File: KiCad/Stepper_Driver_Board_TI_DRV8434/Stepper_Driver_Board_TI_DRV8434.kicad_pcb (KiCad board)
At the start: 4 copper layers, 25 parts, among them J1 Motor Connect, J2 PWR & DATA Connect, J3 Battery Connect, SW1 SW_SPDT_MSM, SW2 SW_SPDT_MSM, U1 DRV8434PWPR, U2 PC817, U4 6N137, U6 PC817

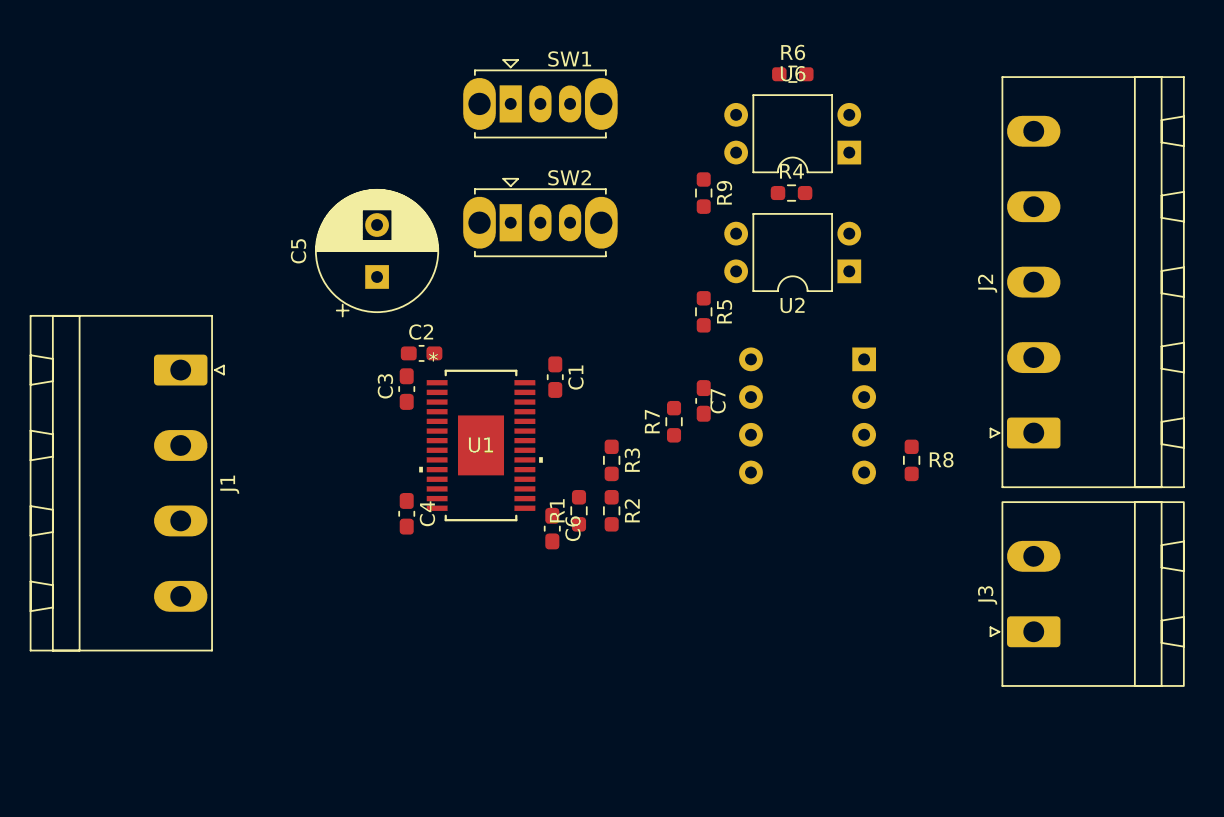
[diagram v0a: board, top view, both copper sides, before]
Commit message: Finished Rough Layout!
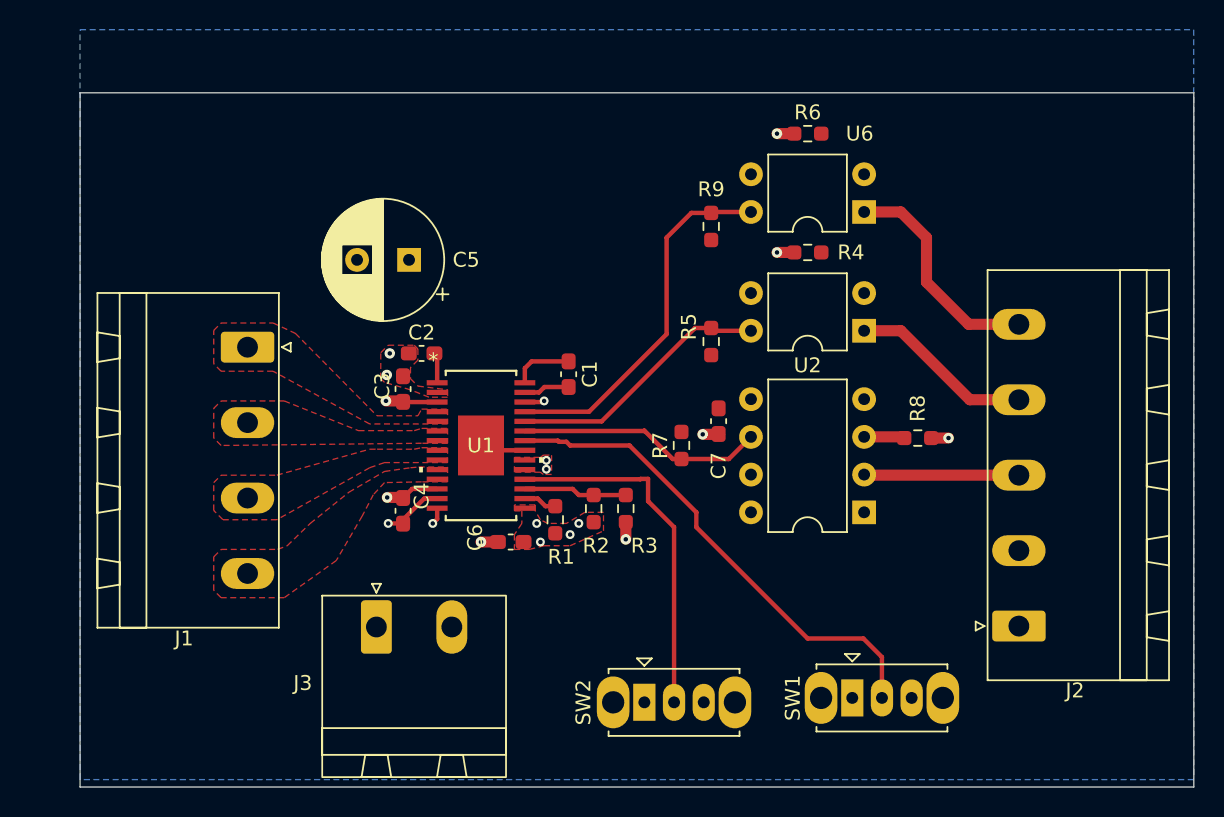
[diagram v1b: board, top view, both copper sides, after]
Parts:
- U4: moved to F.Cu
- moved SW1 46.1 mm to (175.0, 92.0)
- moved J3 44.3 mm to (143.0, 87.2), turned to 0 degrees
- moved SW2 33.5 mm to (161.0, 92.3)
- moved J2 13.0 mm to (186.2, 87.2)
- moved U4 10.3 mm to (175.8, 79.5)
- moved J1 4.76 mm to (134.3, 68.4)
- moved R4 4.15 mm to (172.0, 62.0)
- moved U2 4.12 mm to (175.8, 67.3)
- moved R6 4.12 mm to (172.0, 54.0)
- moved U6 4.12 mm to (175.8, 59.3)
- moved R3 3.39 mm to (159.8, 79.2), turned to 90 degrees
- moved C6 2.94 mm to (152.0, 81.5), turned to 180 degrees
- moved C5 2.44 mm to (145.2, 62.5), turned to 180 degrees
- moved R9 2.30 mm to (165.5, 60.2)
- moved R5 2.06 mm to (165.5, 68.0)
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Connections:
- J2 pad 3: /ENA_ESP -> /PUL_ESP
- J2 pad 5: /PUL_ESP -> /ENA_ESP
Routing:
- net /M1: track 0.00 -> 33.4 mm
- net /ENA: track 0.00 -> 24.6 mm
- net /M0: track 0.00 -> 24.1 mm
- net GND: track 0.00 -> 18.2 mm, vias 0 -> 9
- net /DIR: track 0.00 -> 17.9 mm
- net /PUL: track 0.00 -> 16.6 mm
- net /ENA_ESP: track 0.00 -> 15.3 mm
- net /DIR_ESP: track 0.00 -> 12.3 mm
- net /PUL_ESP: track 0.00 -> 10.4 mm
- net /VREF: track 0.00 -> 6.97 mm
- net +BATT: track 0.00 -> 5.46 mm, vias 0 -> 3
- net /CPH: track 0.00 -> 4.12 mm
- net /CPL: track 0.00 -> 3.10 mm
- net Net-(U4-C): track 0.00 -> 2.73 mm
- net /FAULT: track 0.00 -> 2.26 mm
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- added copper zone on F.Cu, net +5V
- added copper zone on In2.Cu, net +5V
- added copper zone on F.Cu, net +BATT
- added copper zone on In2.Cu, net +BATT
- added copper zone on F.Cu, net /AOUT1
- added copper zone on F.Cu, net /AOUT2
- added copper zone on F.Cu, net /BOUT1
- added copper zone on F.Cu, net /BOUT2
- added copper zone on B.Cu, net GND
- added copper zone on In1.Cu, net GND
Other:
- board outline added: 75 x 46.8 mm
